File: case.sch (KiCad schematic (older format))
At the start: 37 parts

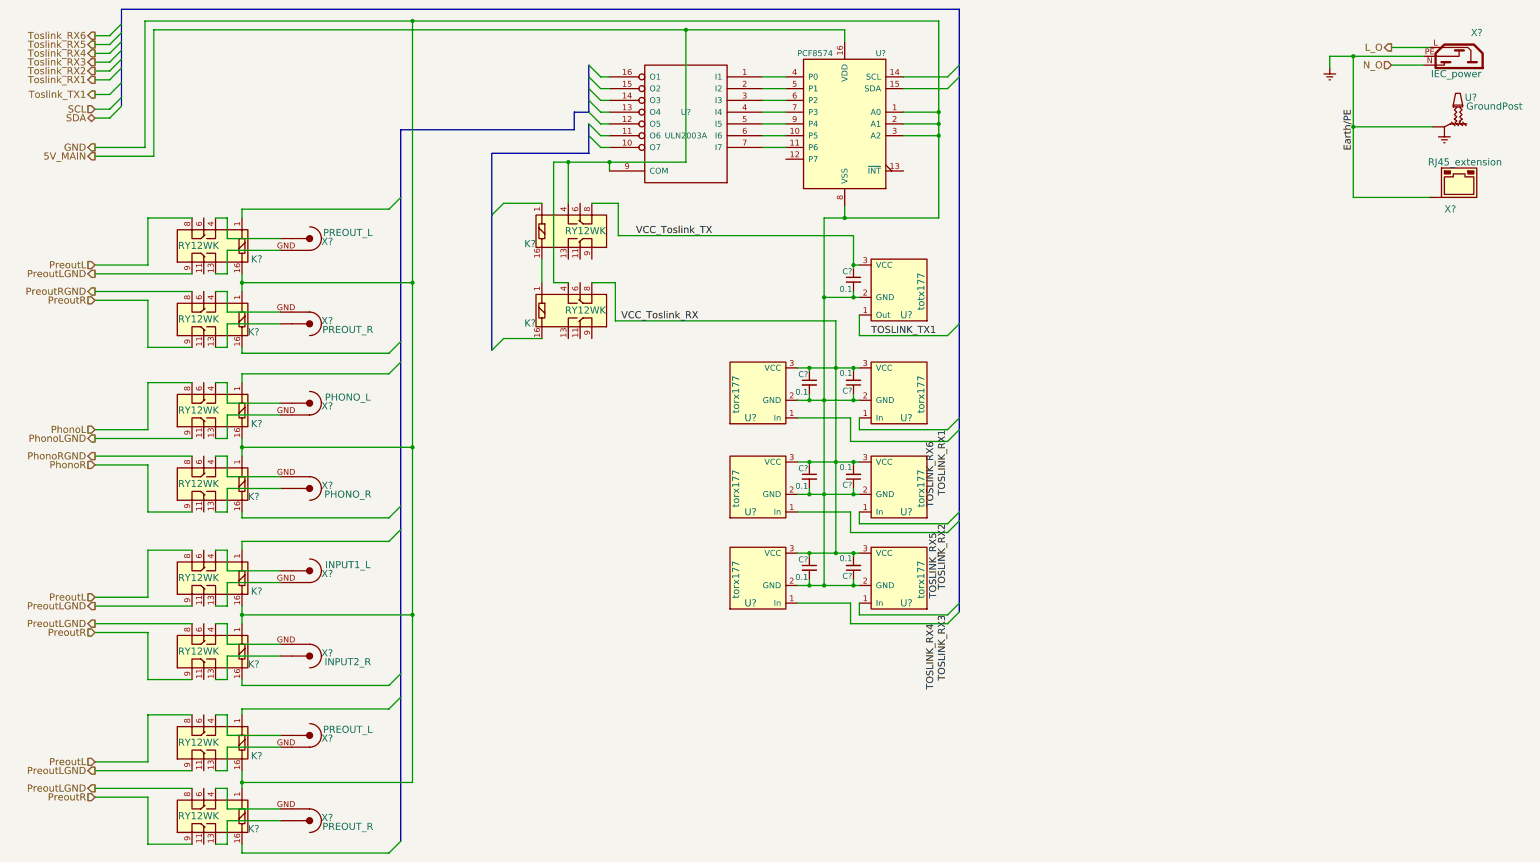
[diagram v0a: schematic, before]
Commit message: daily commit
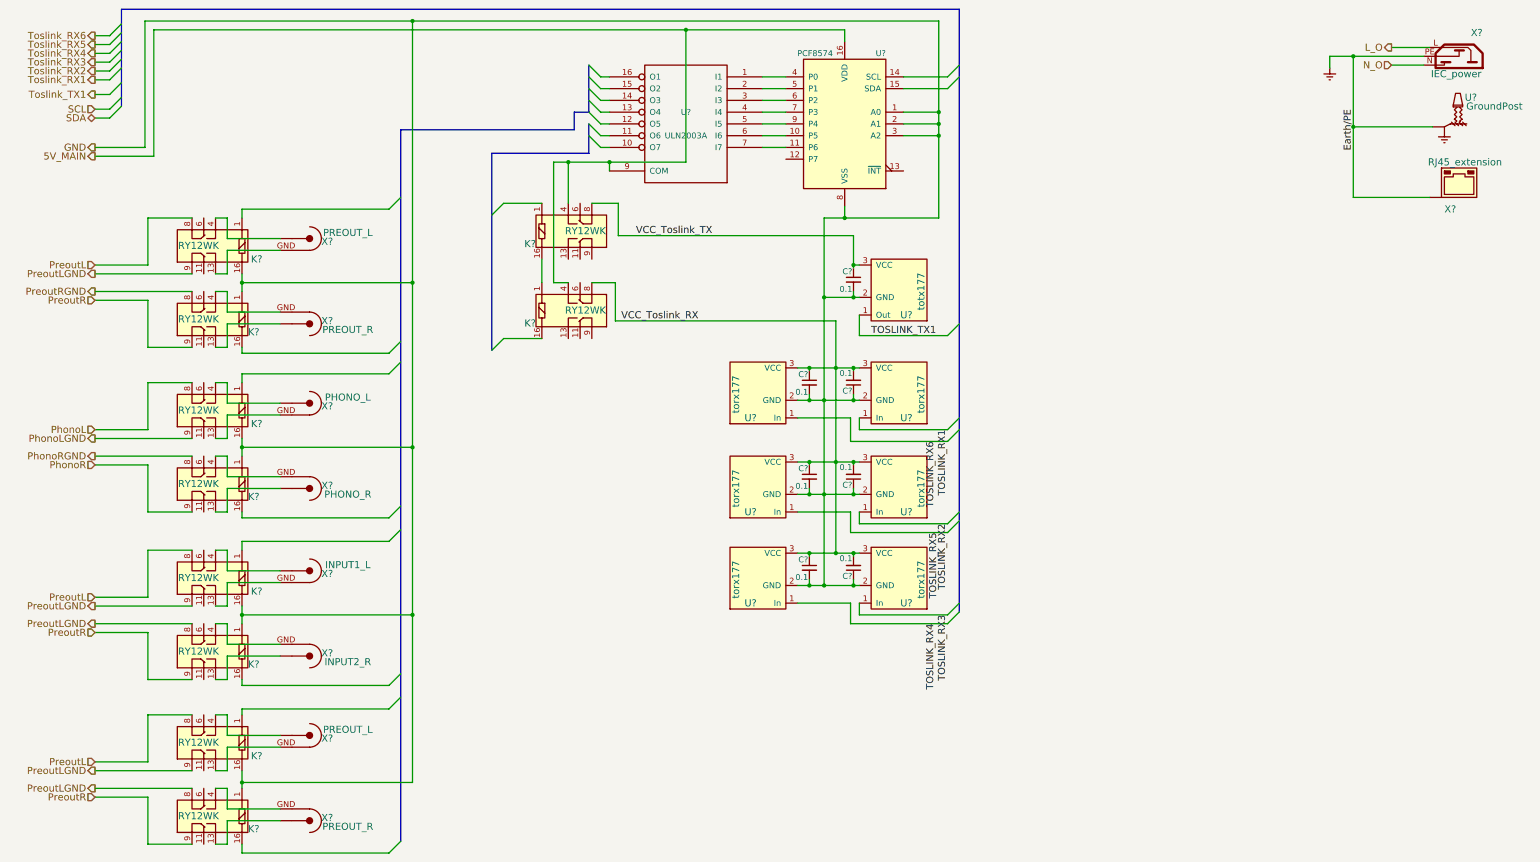
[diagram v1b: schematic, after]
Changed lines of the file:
@@
 	8925 3350 9025 3250
 Wire Wire Line
-	7650 5475 7750 5475
-Wire Wire Line
-	7750 5475 7875 5475
-Wire Wire Line
-	7875 5475 8125 5475
-Wire Wire Line
-	8125 5475 8175 5475
+	7650 5475 8175 5475
 Wire Wire Line
 	7750 5475 7750 5425
 Wire Wire Line
-	7650 5200 7750 5200
-Wire Wire Line
-	7750 5200 7975 5200
-Wire Wire Line
-	7975 5200 8125 5200
-Wire Wire Line
-	8125 5200 8175 5200
+	7650 5200 8175 5200
 Wire Wire Line
 	7750 5200 7750 5225
 Wire Wire Line
-	7650 4700 7750 4700
-Wire Wire Line
-	7750 4700 7875 4700
-Wire Wire Line
-	7875 4700 8125 4700
-Wire Wire Line
-	8125 4700 8175 4700
-Wire Wire Line
-	7650 3900 7750 3900
-Wire Wire Line
-	7750 3900 7875 3900
-Wire Wire Line
-	7875 3900 8125 3900
-Wire Wire Line
-	8125 3900 8175 3900
+	7650 4700 8175 4700
+Wire Wire Line
+	7650 3900 8175 3900
 Wire Wire Line
 	8125 5425 8125 5475
 Connection ~ 8125 5475
 Wire Wire Line
-	7650 4425 7750 4425
-Wire Wire Line
-	7750 4425 7975 4425
-Wire Wire Line
-	7975 4425 8125 4425
-Wire Wire Line
-	8125 4425 8175 4425
-Wire Wire Line
-	7650 3625 7750 3625
-Wire Wire Line
-	7750 3625 7975 3625
-Wire Wire Line
-	7975 3625 8125 3625
-Wire Wire Line
-	8125 3625 8175 3625
+	7650 4425 8175 4425
+Wire Wire Line
+	7650 3625 8175 3625
 Wire Wire Line
 	7750 4700 7750 4650
@@
 	8550 1250 8925 1250
 Wire Wire Line
-	2175 750  6700 750
-Wire Wire Line
-	6700 750  8050 750
-Wire Wire Line
-	8850 2350 8050 2350
-Wire Wire Line
-	8050 2350 7875 2350
+	2175 750  8050 750
+Wire Wire Line
+	8850 2350 7875 2350
 Wire Wire Line
 	1675 800  1800 800
@@
 	1675 1300 1800 1300
 Wire Wire Line
-	8850 675  8850 1450
-Wire Wire Line
-	8850 1450 8850 1550
-Wire Wire Line
-	8850 1550 8850 1650
-Wire Wire Line
-	8850 1650 8850 2350
+	8850 675  8850 2350
 Wire Wire Line
 	8550 1450 8850 1450
@@
 	8850 1650 8550 1650
 Wire Wire Line
-	7975 3225 7975 3625
-Wire Wire Line
-	7975 3625 7975 4425
-Wire Wire Line
-	7975 4425 7975 5200
-Wire Wire Line
-	7875 3025 8125 3025
-Wire Wire Line
-	8125 3025 8175 3025
+	7975 3225 7975 5200
+Wire Wire Line
+	7875 3025 8175 3025
 Wire Wire Line
 	8125 3025 8125 2975
 Wire Wire Line
-	8125 2500 8125 2750
-Wire Wire Line
-	8125 2750 8125 2775
+	8125 2500 8125 2775
 Wire Wire Line
 	8125 2750 8175 2750
 Wire Wire Line
-	7875 2350 7875 3025
-Wire Wire Line
-	7875 3025 7875 3900
-Wire Wire Line
-	7875 3900 7875 4700
-Wire Wire Line
-	7875 4700 7875 5475
+	7875 2350 7875 5475
 Connection ~ 8125 3025
 Connection ~ 8850 1650
@@
 $EndComp
 Wire Bus Line
-	1900 575  1900 700
-Wire Bus Line
-	1900 700  1900 775
-Wire Bus Line
-	1900 775  1900 850
-Wire Bus Line
-	1900 850  1900 925
-Wire Bus Line
-	1900 925  1900 1000
-Wire Bus Line
-	1900 1000 1900 1075
-Wire Bus Line
-	1900 1075 1900 1200
-Wire Bus Line
-	1900 1200 1900 1325
-Wire Bus Line
-	1900 1325 1900 1400
+	1900 575  1900 1400
 Wire Wire Line
 	1675 1750 2100 1750
@@
 	12975 1050 12700 1050
 Wire Wire Line
-	12175 975  12375 975
-Wire Wire Line
-	12375 975  12975 975
+	12175 975  12975 975
 Wire Wire Line
 	12175 975  12175 1075
 Wire Wire Line
-	12375 975  12375 1575
-Wire Wire Line
-	12375 1575 12375 2175
+	12375 975  12375 2175
 Wire Wire Line
 	12375 1575 13050 1575
@@
 	8925 5800 9025 5700
 Wire Bus Line
-	9025 575  9025 1050
-Wire Bus Line
-	9025 1050 9025 1150
-Wire Bus Line
-	9025 1150 9025 3250
-Wire Bus Line
-	9025 3250 9025 4050
-Wire Bus Line
-	9025 4050 9025 4150
-Wire Bus Line
-	9025 4150 9025 4850
-Wire Bus Line
-	9025 4850 9025 4925
-Wire Bus Line
-	9025 4925 9025 5625
-Wire Bus Line
-	9025 5625 9025 5700
+	9025 575  9025 5700
 Wire Wire Line
 	8175 4050 8175 4150
@@
 $EndComp
 Wire Wire Line
-	2925 2825 2925 2900
-Wire Wire Line
-	2925 2900 2925 2975
+	2925 2825 2925 2975
 Wire Wire Line
 	3250 3150 2800 3150
@@
 $EndComp
 Wire Wire Line
-	2925 4225 2925 4300
-Wire Wire Line
-	2925 4300 2925 4375
+	2925 4225 2925 4375
 Wire Wire Line
 	3250 4550 2800 4550
@@
 $EndComp
 Wire Wire Line
-	2925 5650 2925 5725
-Wire Wire Line
-	2925 5725 2925 5800
+	2925 5650 2925 5800
 Wire Wire Line
 	3250 5975 2800 5975
@@
 $EndComp
 Wire Wire Line
-	2925 7050 2925 7150
-Wire Wire Line
-	2925 7150 2925 7200
+	2925 7050 2925 7200
 Wire Wire Line
 	3250 7375 2800 7375
@@
 	6050 1550 5975 1550
 Wire Bus Line
-	5875 1050 5875 1150
+	5875 1050 5875 1450
 Wire Bus Line
-	5875 1150 5875 1250
-Wire Bus Line
-	5875 1250 5875 1350
-Wire Bus Line
-	5875 1350 5875 1450
-Wire Bus Line
-	4275 1600 4275 2175
-Wire Bus Line
-	4275 2175 4275 3400
-Wire Bus Line
-	4275 3400 4275 3575
-Wire Bus Line
-	4275 3575 4275 4800
-Wire Bus Line
-	4275 4800 4275 5000
-Wire Bus Line
-	4275 5000 4275 6225
-Wire Bus Line
-	4275 6225 4275 6425
-Wire Bus Line
-	4275 6425 4275 7650
+	4275 1600 4275 7650
 Entry Wire Line
 	4175 3500 4275 3400
@@
 	2925 2900 4375 2900
 Wire Wire Line
-	4375 675  4375 2900
-Wire Wire Line
-	4375 2900 4375 4300
-Wire Wire Line
-	4375 4300 4375 5725
-Wire Wire Line
-	4375 5725 4375 7150
+	4375 675  4375 7150
 Connection ~ 2925 2900
 Wire Wire Line
@@
 $EndComp
 Wire Wire Line
-	2100 675  4375 675
-Wire Wire Line
-	4375 675  8850 675
+	2100 675  8850 675
 $Comp
 L RY12WK K?
@@
 	6050 1875 6050 1950
 Wire Wire Line
-	5575 1875 5700 1875
-Wire Wire Line
-	5700 1875 6050 1875
-Wire Wire Line
-	6050 1875 6700 1875
+	5575 1875 6700 1875
 Wire Wire Line
 	6700 1875 6700 750
@@
 	6050 1750 5975 1750
 Wire Bus Line
-	5875 1550 5875 1650
-Wire Bus Line
-	5875 1650 5875 1800
+	5875 1550 5875 1800
 Wire Bus Line
 	5875 1800 5050 1800
 Wire Bus Line
-	5050 1800 5050 2325
-Wire Bus Line
-	5050 2325 5050 3475
+	5050 1800 5050 3475
 Entry Wire Line
 	5050 3475 5150 3375
